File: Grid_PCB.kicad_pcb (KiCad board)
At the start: 2 copper layers, 223.2 x 22 mm, 42 parts, among them J1 Conn_01x04_Female, J10 LED_Conn, J11 Power_Conn, J2 Conn_01x04_Female, J3 Conn_01x04_Female, J4 Conn_01x04_Female, J5 Conn_01x04_Female, J6 Conn_01x04_Female, J7 Conn_01x04_Female, J8 Conn_01x04_Female, J9 ESP_Conn, U1 SN74HC151N

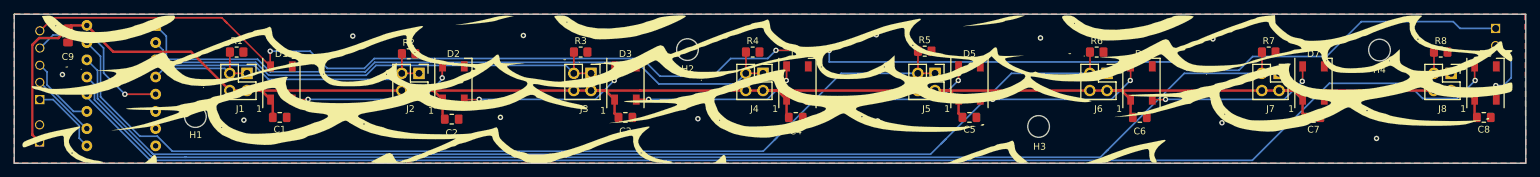
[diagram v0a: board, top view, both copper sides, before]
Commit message: wave 4
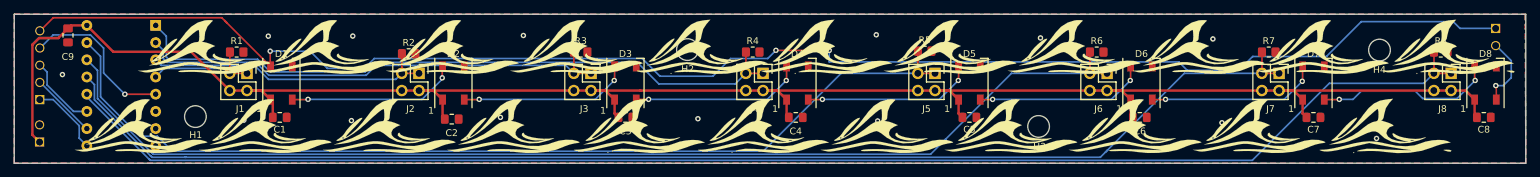
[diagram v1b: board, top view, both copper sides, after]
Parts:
- removed the G*** at (154.3, 94.9)
- added G***: LOGO, grid:wave_pattern_4, F.Cu at (153.2, 100.0)
- added G***: LOGO, grid:wave_pattern_4, F.Cu at (162.5, 88.3)
